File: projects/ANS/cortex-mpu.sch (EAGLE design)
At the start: 7 parts, among them IC1 LM1117MPX-3.3, U1 AT32UC3B164-AUT

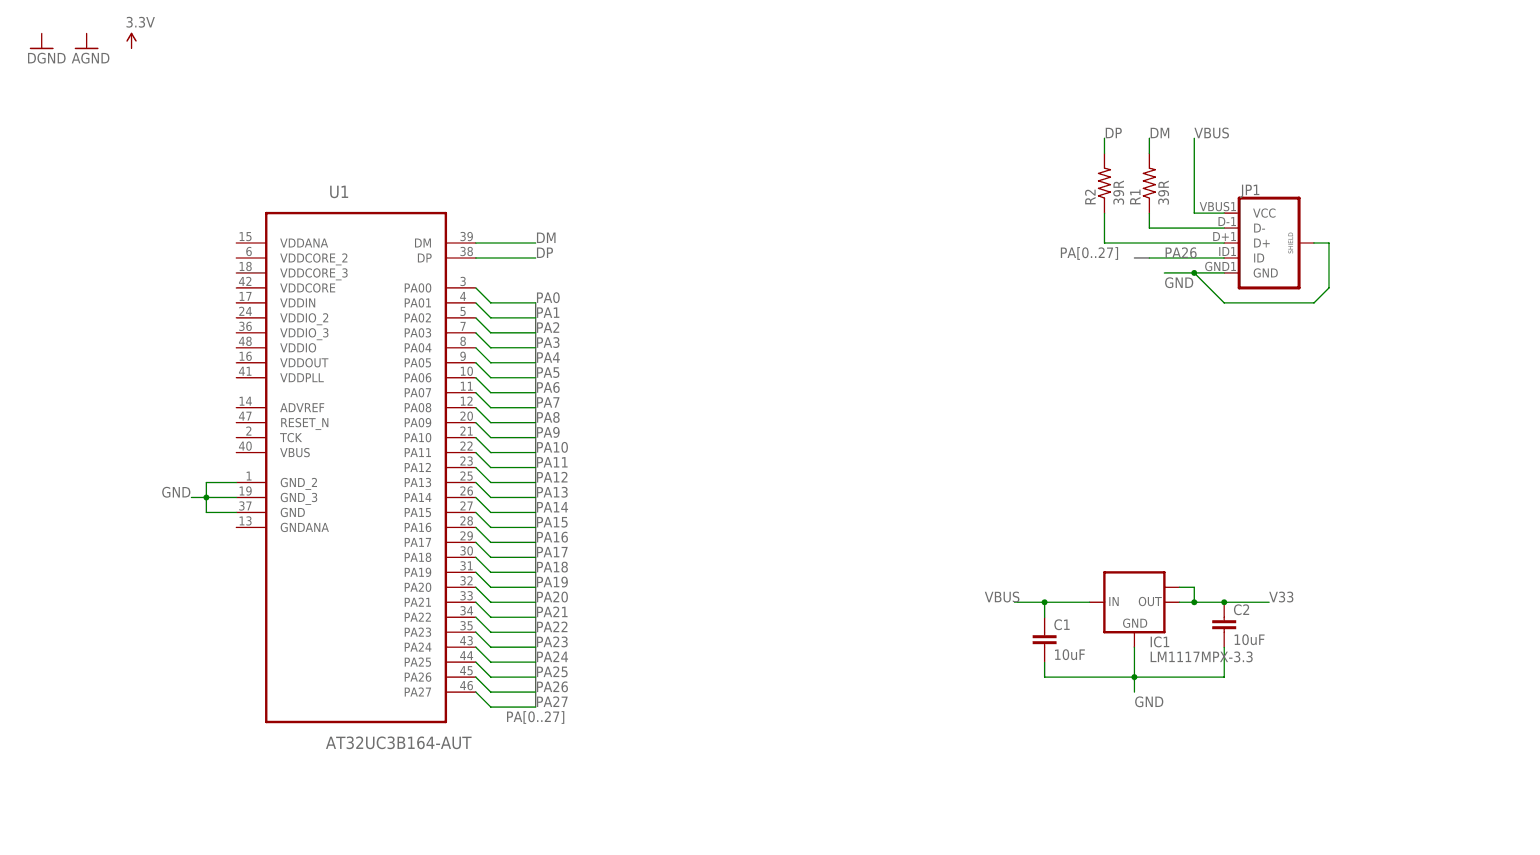
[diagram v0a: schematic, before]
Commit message: Various Groups
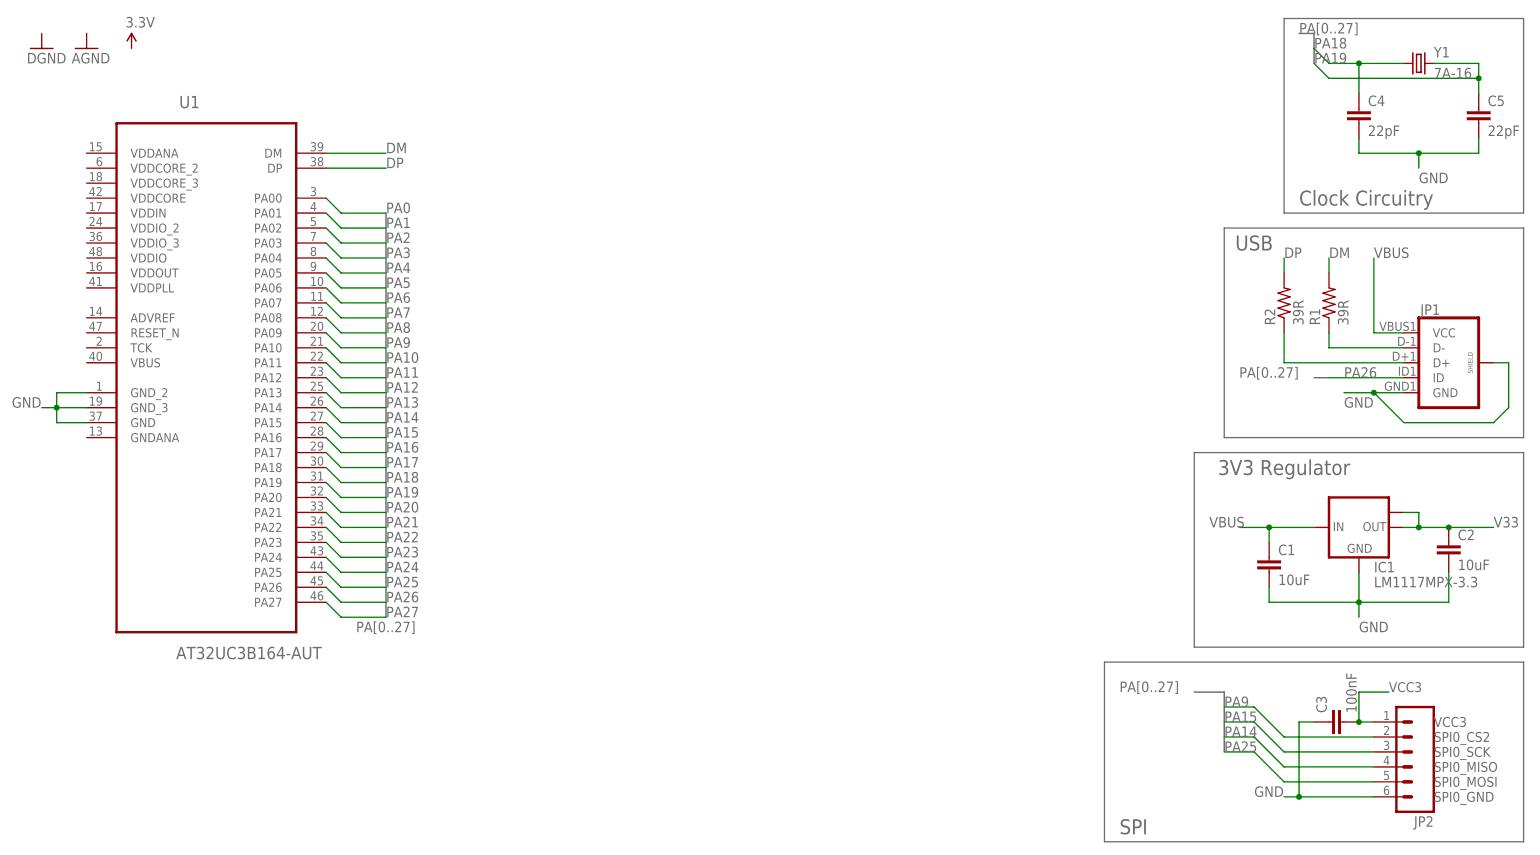
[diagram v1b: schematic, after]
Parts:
- added C3: 100nF, SparkFun-Passives:CAP0603-CAP
- added C4, C5: 22pF, SparkFun-Passives:CAP0603-CAP
- added JP2: (no value), SparkFun-Connectors:M06LOCK_LONGPADS
- added Y1: 7A-16, SparkFun-FreqCtrl:CRYSTALTXC-7A
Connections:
- new net VCC3: C3.2, JP2.1
- net GND: now also C3.1, C4.2, C5.2, JP2.6
- net PA14: now also JP2.4
- net PA15: now also JP2.3
- net PA18: now also C4.1, Y1.1
- net PA19: now also C5.1, Y1.2
- net PA25: now also JP2.5
- net PA9: now also JP2.2
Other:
- note added: "3V3 Regulator"
- note added: "Clock Circuitry"
- note added: "SPI"
- note added: "SPI0_CS2"
- note added: "SPI0_GND"
- note added: "SPI0_MISO"
- note added: "SPI0_MOSI"
- note added: "SPI0_SCK"
- note added: "USB"
- note added: "VCC3"
- moved on the sheet: C1, C2, IC1, JP1, R1, R2, U1
